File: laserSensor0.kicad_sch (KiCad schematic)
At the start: 7 parts, among them U601 LSM6DSM

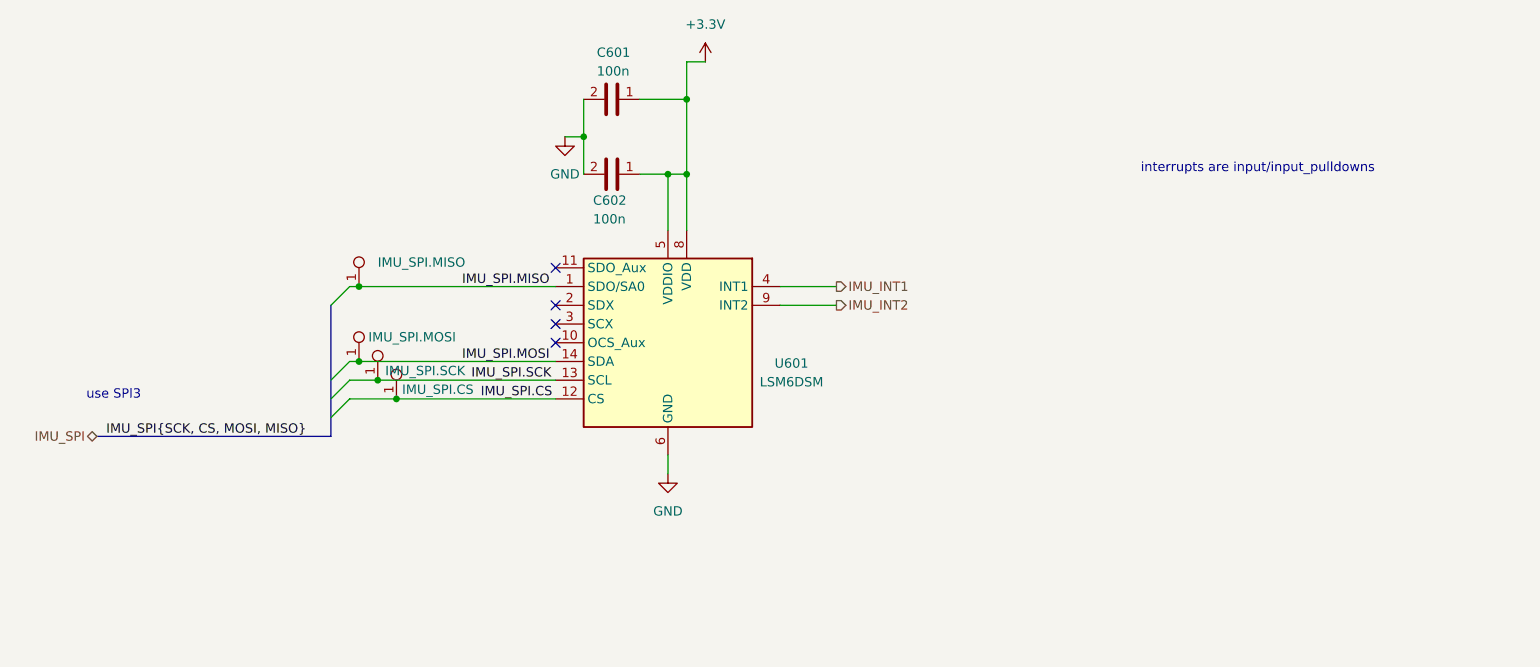
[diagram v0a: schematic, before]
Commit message: preliminary schematic
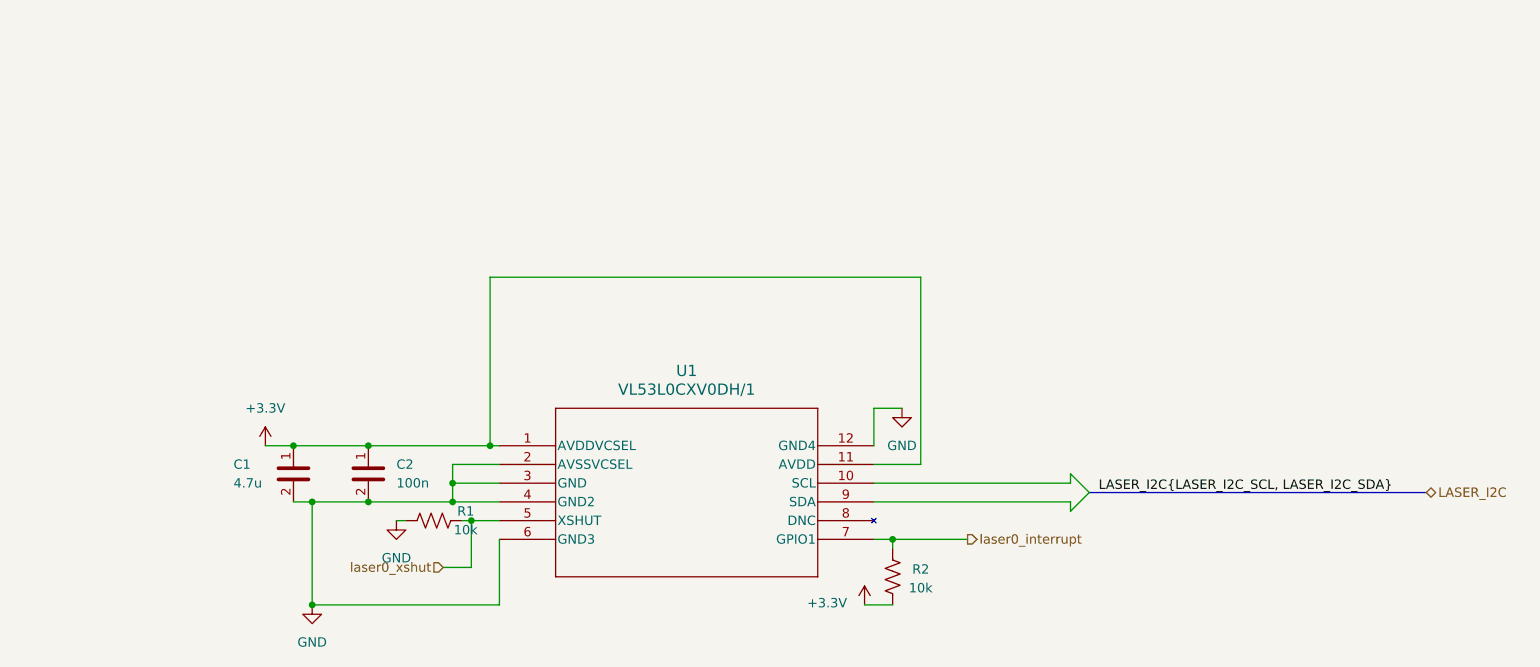
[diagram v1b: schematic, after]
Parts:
- removed C601, C602: 100n, Capacitor_SMD:C_0603_1608Metric_Pad1.08x0.95mm_HandSolder, symbol bfr_capacitors:06035C104KAT2A
- removed TP601: IMU_SPI.MISO, bfr_utilities:TestPoint_Keystone_5019_Miniature, symbol bfr_master:SMD_Test_Point
- removed TP602: IMU_SPI.MOSI, bfr_utilities:TestPoint_Keystone_5019_Miniature, symbol bfr_master:SMD_Test_Point
- removed TP603: IMU_SPI.SCK, bfr_utilities:TestPoint_Keystone_5019_Miniature, symbol bfr_master:SMD_Test_Point
- removed TP604: IMU_SPI.CS, bfr_utilities:TestPoint_Keystone_5019_Miniature, symbol bfr_master:SMD_Test_Point
- removed U601: LSM6DSM, Package_LGA:LGA-14_3x2.5mm_P0.5mm_LayoutBorder3x4y, symbol Sensor_Motion:LSM6DSM
- added C1: 4.7u, Capacitor_SMD:C_0805_2012Metric_Pad1.18x1.45mm_HandSolder, symbol bfr_capacitors:KGM21AR51A475KU
- added C2: 100n, Capacitor_SMD:C_0603_1608Metric_Pad1.08x0.95mm_HandSolder, symbol bfr_capacitors:06035C104KAT2A
- added R1, R2: 10k, Resistor_SMD:R_0603_1608Metric_Pad0.98x0.95mm_HandSolder, symbol bfr_resistors:RMCF0603FT10K0
- added U1: VL53L0CXV0DH/1, LGA12_STM, symbol VL53L0CXV0DH/1:VL53L0CXV0DH_1
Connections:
- net +3.3V: now also C1.1, C2.1, R2.2, U1.1 (AVDDVCSEL), U1.11 (AVDD)
- net GND: now also C1.2, C2.2, R1.1, U1.12 (GND4), U1.2 (AVSSVCSEL), U1.3 (GND), U1.4 (GND2), U1.6 (GND3)
- new net laser0_interrupt: R2.1, U1.7 (GPIO1)
- new net laser0_xshut: R1.2, U1.5 (XSHUT)
- no-connect marks 4 -> 0
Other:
- note removed: "interrupts are input/input_pulldowns"
- note removed: "use SPI3"
